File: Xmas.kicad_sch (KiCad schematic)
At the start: 24 parts, among them IC1 STM32C011F6, IC2 TP4056-42, SW1 BZCN_TSA007A1518B03

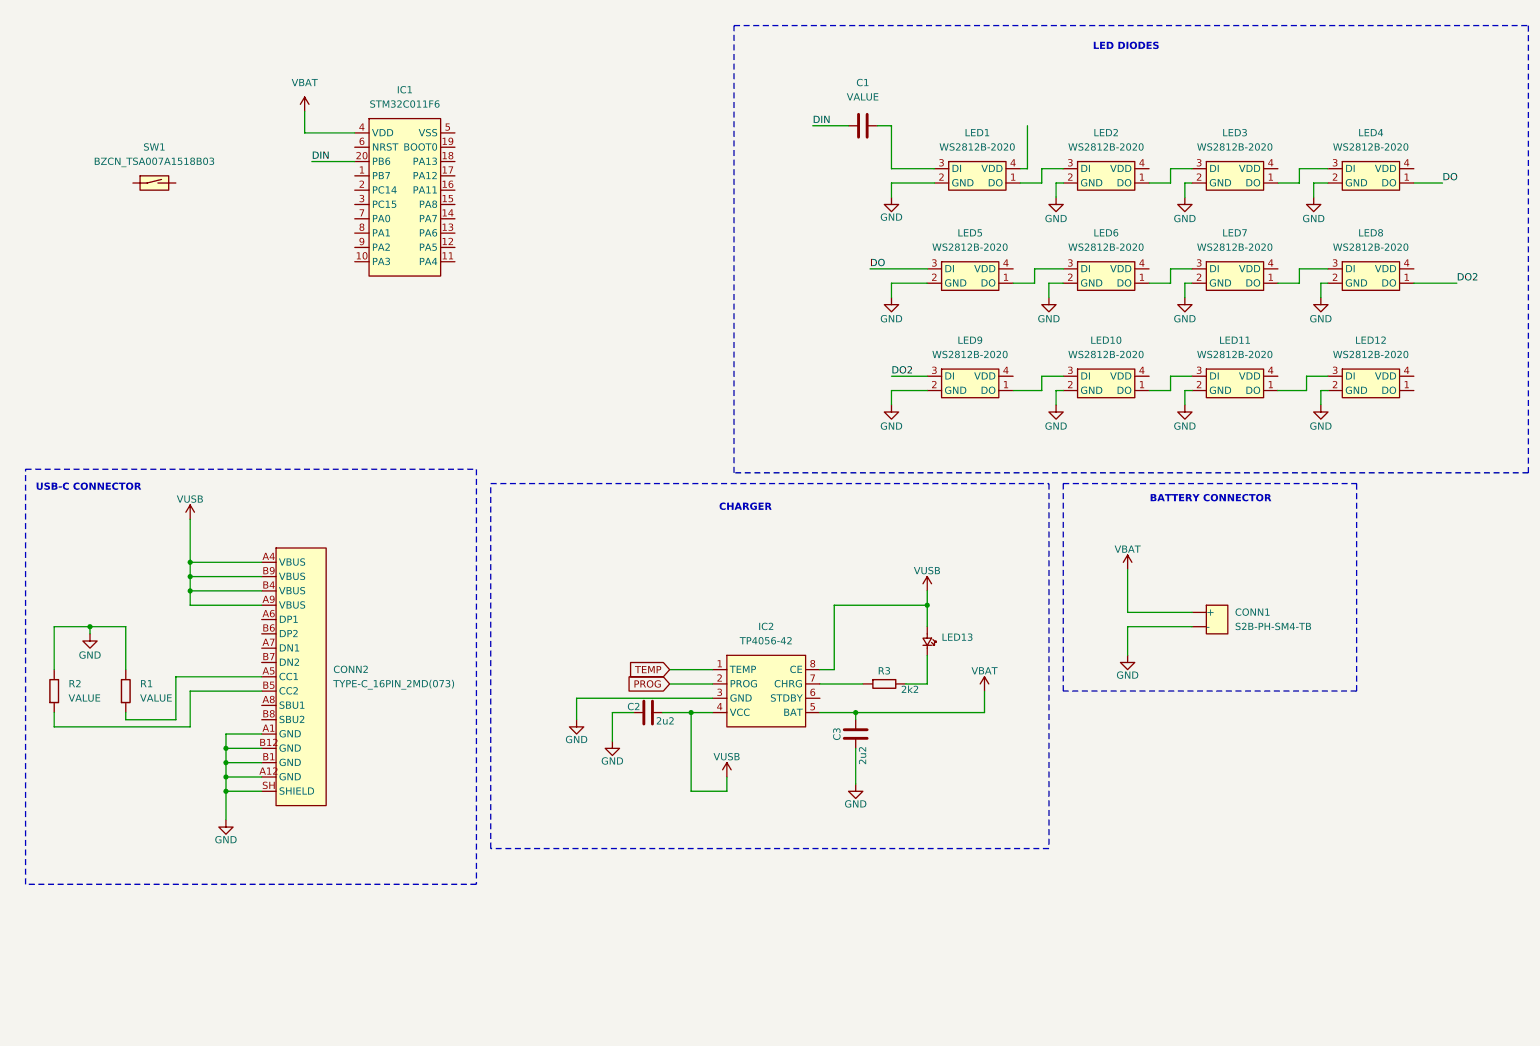
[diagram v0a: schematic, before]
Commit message: The schematic is complete
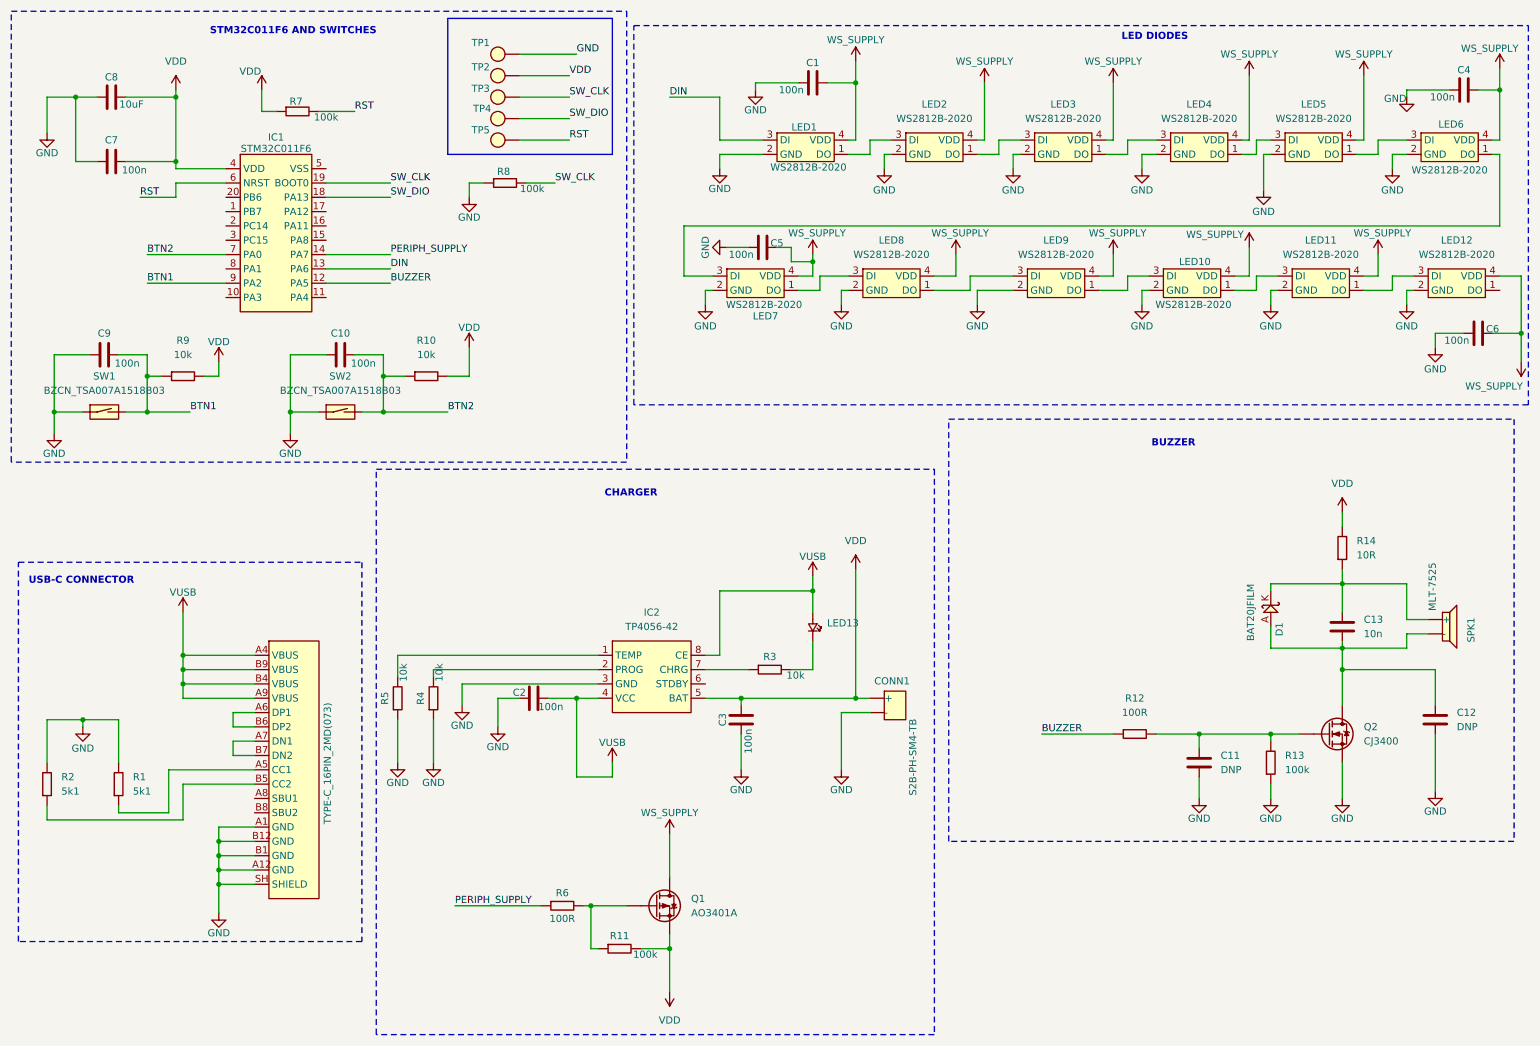
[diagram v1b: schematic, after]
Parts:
- added C10, C4, C5, C6, C7, C9: 100n, BornaKiCad:C0603, symbol BornaLibrary:C0603
- added C11, C12: DNP, BornaKiCad:C0603, symbol BornaLibrary:C0603
- added C13: 10n, BornaKiCad:C0603, symbol BornaLibrary:C0603
- added C8: 10uF, BornaKiCad:C1206, symbol BornaLibrary:C1206
- added D1: BAT20JFILM, BornaKiCad:SOD323, symbol BornaLibrary:BAT20JFILM
- added Q1: AO3401A, BornaKiCad:SOT-23-3L, symbol BornaLibrary:AO3401A
- added Q2: CJ3400, BornaKiCad:SOT-23-3L, symbol BornaLibrary:CJ3400
- added R10, R4, R5, R9: 10k, BornaKiCad:R0603, symbol BornaLibrary:R0603
- added R11, R13, R7, R8: 100k, BornaKiCad:R0603, symbol BornaLibrary:R0603
- added R12, R6: 100R, BornaKiCad:R0603, symbol BornaLibrary:R0603
- added R14: 10R, BornaKiCad:R1206, symbol BornaLibrary:R1206
- added SPK1: MLT-7525, BornaKiCad:MTL-7525, symbol BornaLibrary:MLT-7525
- added SW2: BZCN_TSA007A1518B03, BornaKiCad:TSA007A1518B03, symbol BornaLibrary:BZCN_TSA007A1518B03
- added TP1, TP2, TP3, TP4, TP5: ~, BornaKiCad:TP-1_5mm, symbol BornaLibrary:TP-1_5mm
- C1: value VALUE -> 100n; footprint BornaKiCad:C1206 -> BornaKiCad:C0603; symbol BornaLibrary:C1206 -> BornaLibrary:C0603
- C2, C3: value 2u2 -> 100n
- R1, R2: value VALUE -> 5k1
- R3: value 2k2 -> 10k
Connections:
- net DIN: now also IC1.13 (PA6), LED1.3 (DI); no longer C1.1, IC1.20 (PB6)
- net GND: now also C1.1, SW1.1 (SW1), C10.1, C11.1, C12.1, C4.1, C5.1, C6.1, C7.1, C8.1, C9.1, Q2.3 (S), R13.1, R4.1, R5.1, R8.1, SW2.1 (SW1), TP1.1 (TP)
- net WS_SUPPLY: now reaches LED7.4 (VDD)
- net WS_SUPPLY: now also C1.2, LED1.4 (VDD), LED10.4 (VDD), LED11.4 (VDD), LED12.4 (VDD), LED2.4 (VDD), LED3.4 (VDD), LED4.4 (VDD), LED5.4 (VDD), LED6.4 (VDD), LED8.4 (VDD), LED9.4 (VDD), C4.2, C5.2, C6.2, Q1.2 (D)
- net BUZZER: now reaches IC1.12 (PA5)
- net BUZZER: now also R12.1
- net PERIPH_SUPPLY: now reaches IC1.14 (PA7)
- net PERIPH_SUPPLY: now also R6.1
- net SW_DIO: now reaches IC1.18 (PA13)
- net SW_DIO: now also TP4.1 (TP)
- net SW_CLK: now reaches IC1.19 (BOOT0)
- net SW_CLK: now also R8.2, TP3.1 (TP)
- net RST: now reaches IC1.6 (NRST)
- net RST: now also R7.2, TP5.1 (TP)
- net BTN2: now reaches IC1.7 (PA0)
- net BTN2: now also C10.2, R10.1, SW2.2 (SW2)
- net BTN1: now reaches IC1.9 (PA2)
- net BTN1: now also SW1.2 (SW2), C9.2, R9.1
- net at CONN2.A6 (DP1): now also CONN2.B6 (DP2)
- net at CONN2.A7 (DN1): now also CONN2.B7 (DN2)
- net DO: no longer names the net of LED4.1 (DO), LED5.3 (DI)
- net DO2: no longer names the net of LED8.1 (DO), LED9.3 (DI)
- net PROG: no longer names the net of IC2.2 (PROG)
- net PROG: now also R4.2
- net TEMP: no longer names the net of IC2.1 (TEMP)
- net TEMP: now also R5.2
- net VBAT renamed VDD
- net VDD: now also C7.2, C8.2, Q1.3 (S), R10.2, R11.2, R14.2, R7.1, R9.2, TP2.1 (TP)
- new net: Q1.1 (G), R11.1, R6.2
- new net: C12.2, C13.1, D1.A, Q2.2 (D), SPK1.-
- new net: C13.2, D1.K, R14.1, SPK1.+
- new net: C11.2, Q2.1 (G), R12.2, R13.2
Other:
- note added: "BUZZER"
- note added: "STM32C011F6 AND SWITCHES"
- note removed: "BATTERY CONNECTOR"
- moved on the sheet: C1, C2, C3, CONN1, IC1, IC2, LED1, LED10, LED11, LED12, LED13, LED2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
